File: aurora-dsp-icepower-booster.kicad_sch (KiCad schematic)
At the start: 232 parts, among them J1 XLR_IN_1, J10 XLR3_OUT, J11 XLR3_OUT, J12 XLR3_OUT, J13 24V DC, J2 XLR_IN_2, J3 XLR_IN_3, J4 XLR_IN_4, J5 XLR_IN_5, J6 XLR_IN_6, J7 XLR3_OUT, J8 XLR3_OUT, J9 XLR3_OUT, SW1 Gain CH1, SW2 Gain CH2, SW3 Gain CH3, SW4 Gain CH4, SW5 Gain CH5, SW6 Gain CH6, U1 LM4562, U10 LM4562, U11 LM4562, U12 LM4562, U13 TEL5-2422, U14 ADP7118ARDZ-11, U15 ADP7182AUJZ-11, U2 LM4562, U3 LM4562, U4 LM4562, U5 LM4562, U6 LM4562, U7 LM4562, U8 LM4562, U9 LM4562

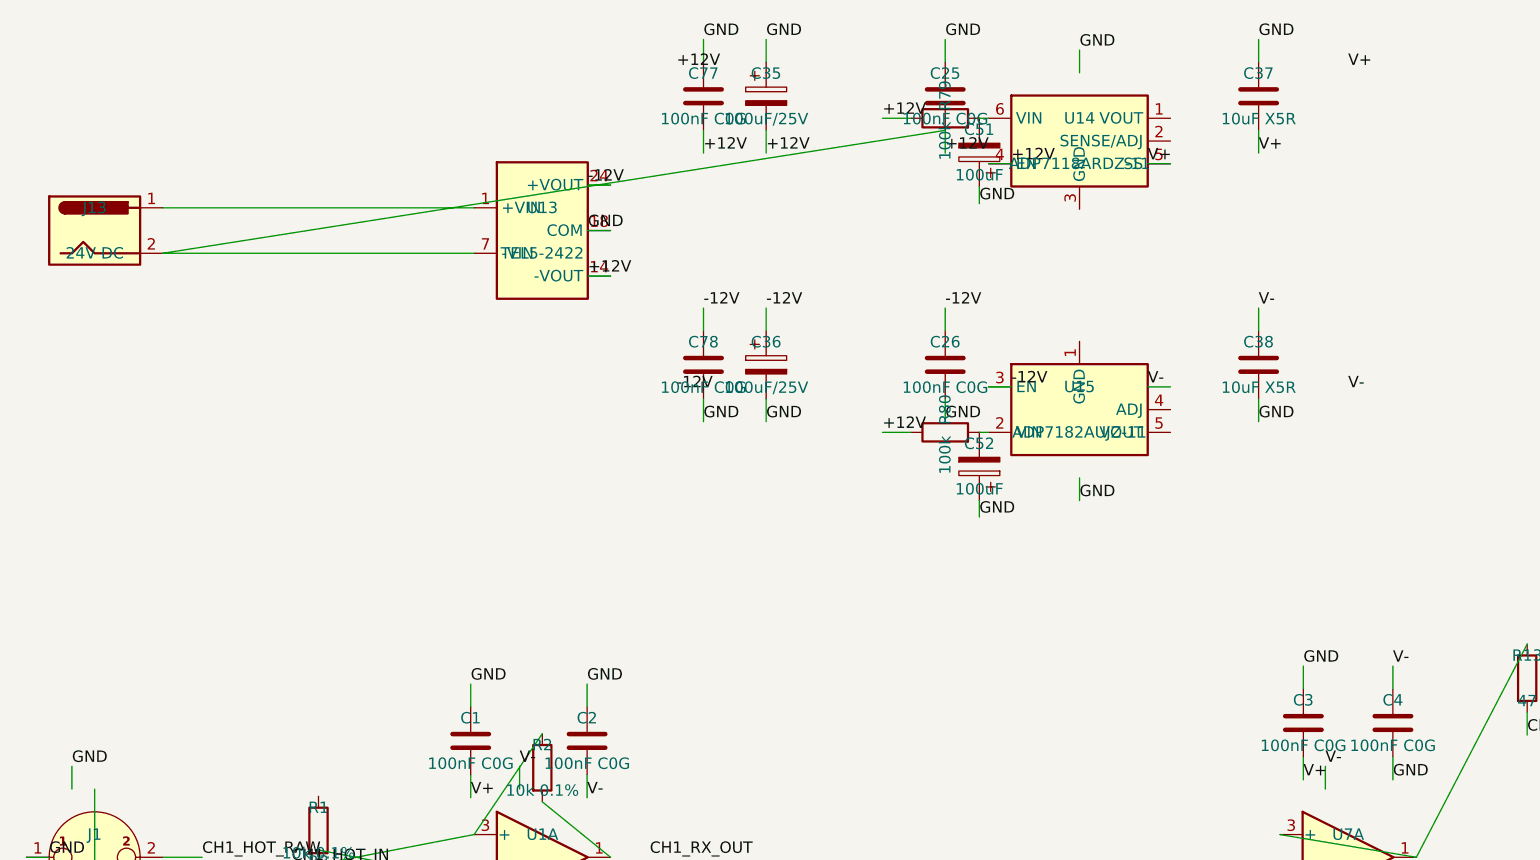
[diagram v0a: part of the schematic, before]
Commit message: chore: 🔄 empty code changes
* No code changes were made in this commit.
* This serves as a placeholder for future updates.
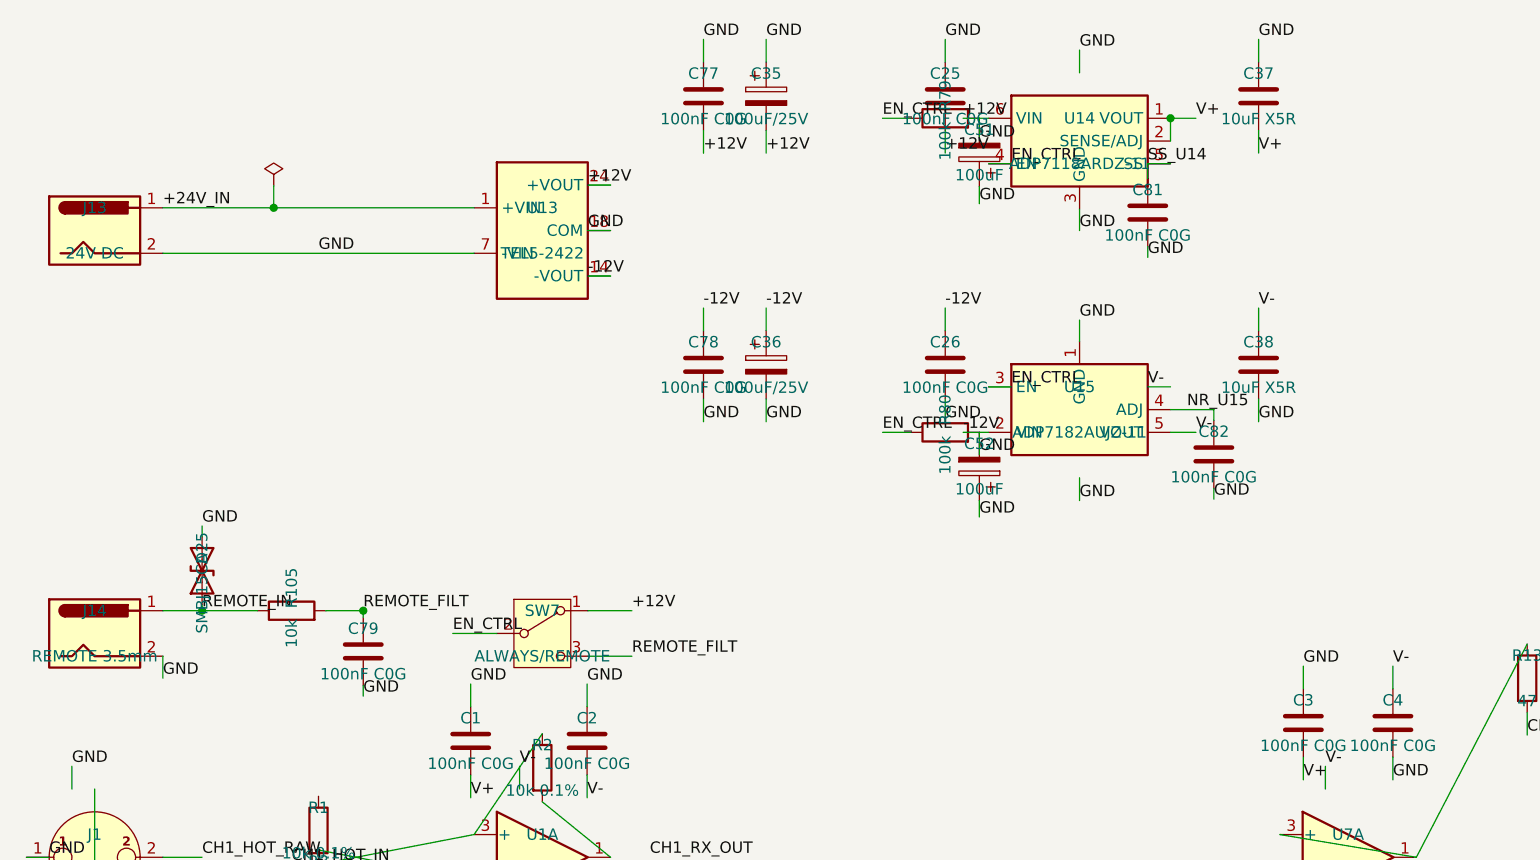
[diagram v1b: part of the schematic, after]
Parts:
- added C79, C81, C82: 100nF C0G, Capacitor_SMD:C_0805_2012Metric, symbol Device:C
- added D25: SMBJ15CA, Diode_SMD:D_SMB, symbol Device:D_TVS
- added J14: REMOTE 3.5mm, Connector_Audio:AudioJack2_Ground_Switch_Lumberg_1503_09, symbol Connector:Barrel_Jack
- added R105: 10k, Resistor_SMD:R_0805_2012Metric, symbol Device:R
- added SW7: ALWAYS/REMOTE, Connector_PinHeader_2.54mm:PinHeader_1x03_P2.54mm_Vertical, symbol Switch:SW_SPDT
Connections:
- net +12V: now also U13.24 (+VOUT), U14.6 (VIN), SW7.1 (A); no longer J13.2, R79.1, R80.1, U13.14 (-VOUT), U13.7 (-VIN), U14.4 (EN)
- net -12V: now also U13.14 (-VOUT), U15.2 (VIN); no longer U13.24 (+VOUT), U15.3 (EN)
- net GND: now also C51.2, C52.2, J13.2, R79.2, R80.2, U13.7 (-VIN), U14.3 (GND), U14.7 (GND), U15.1 (GND), C79.2, C81.2, C82.2, D25.2 (A2), J14.2
- net V+: now also U14.1 (VOUT), U14.2 (SENSE/ADJ); no longer U14.5 (SS)
- net V-: now also U15.5 (VOUT)
- net +24V_IN: now reaches J13.1, U13.1 (+VIN)
- net NR_U15: now reaches U15.4 (ADJ)
- net NR_U15: now also C82.1
- new net EN_CTRL: R79.1, R80.1, SW7.2 (B), U14.4 (EN), U15.3 (EN)
- new net REMOTE_FILT: C79.1, R105.2, SW7.3 (C)
- new net REMOTE_IN: D25.1 (A1), J14.1, R105.1
- new net SS_U14: C81.1, U14.5 (SS)
